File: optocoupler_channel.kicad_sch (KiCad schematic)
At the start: 22 parts, among them Q1 MMBT5551 200-300, Q2 MMBT5551 200-300, Q3 MMBT5401 200-300, Q4 MMBT5551 200-300, Q5 MMBT5551 200-300, U3 LTV-217-B-G, U5 LTV-217-B-G, U6 LTV-217-B-G

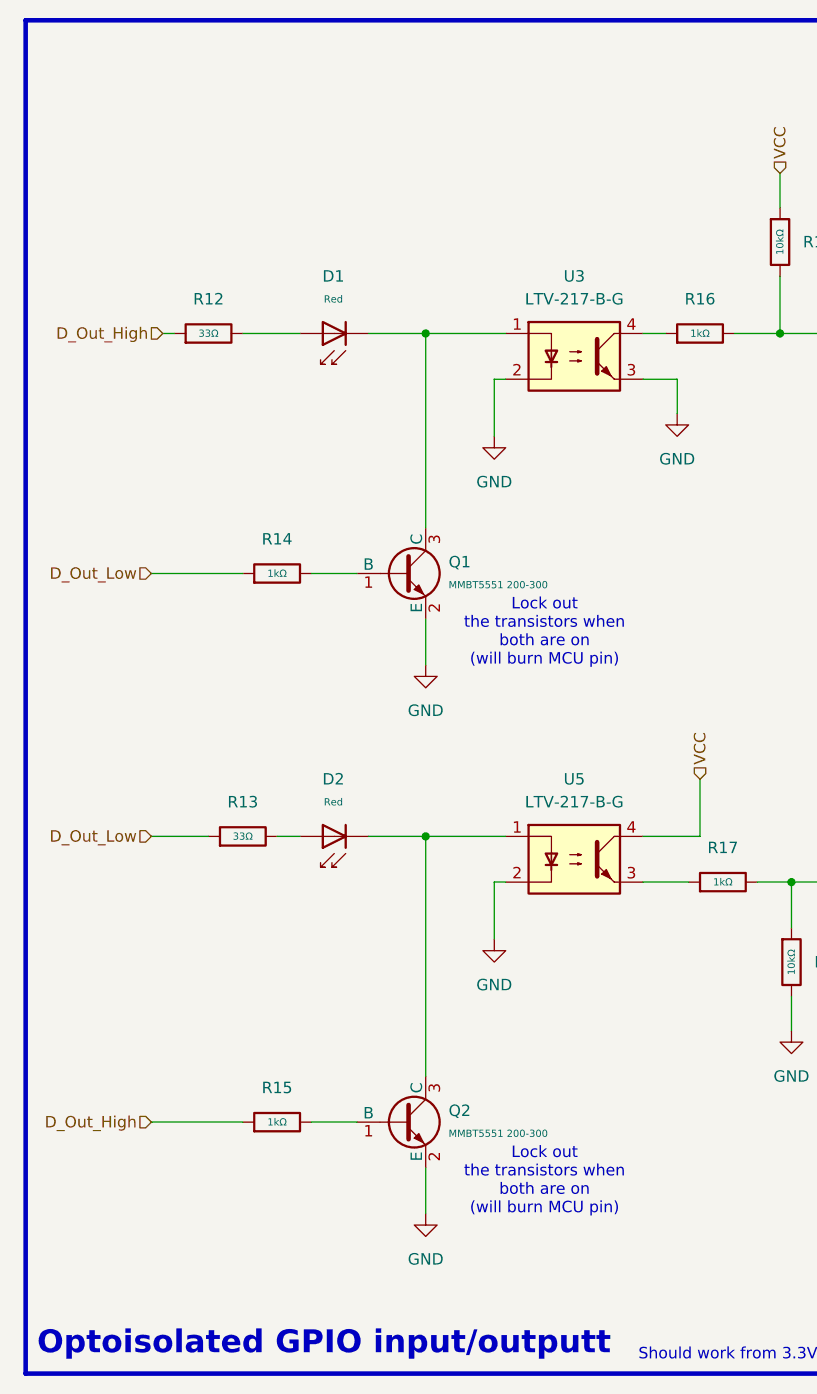
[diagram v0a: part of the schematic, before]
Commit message: routing impossible
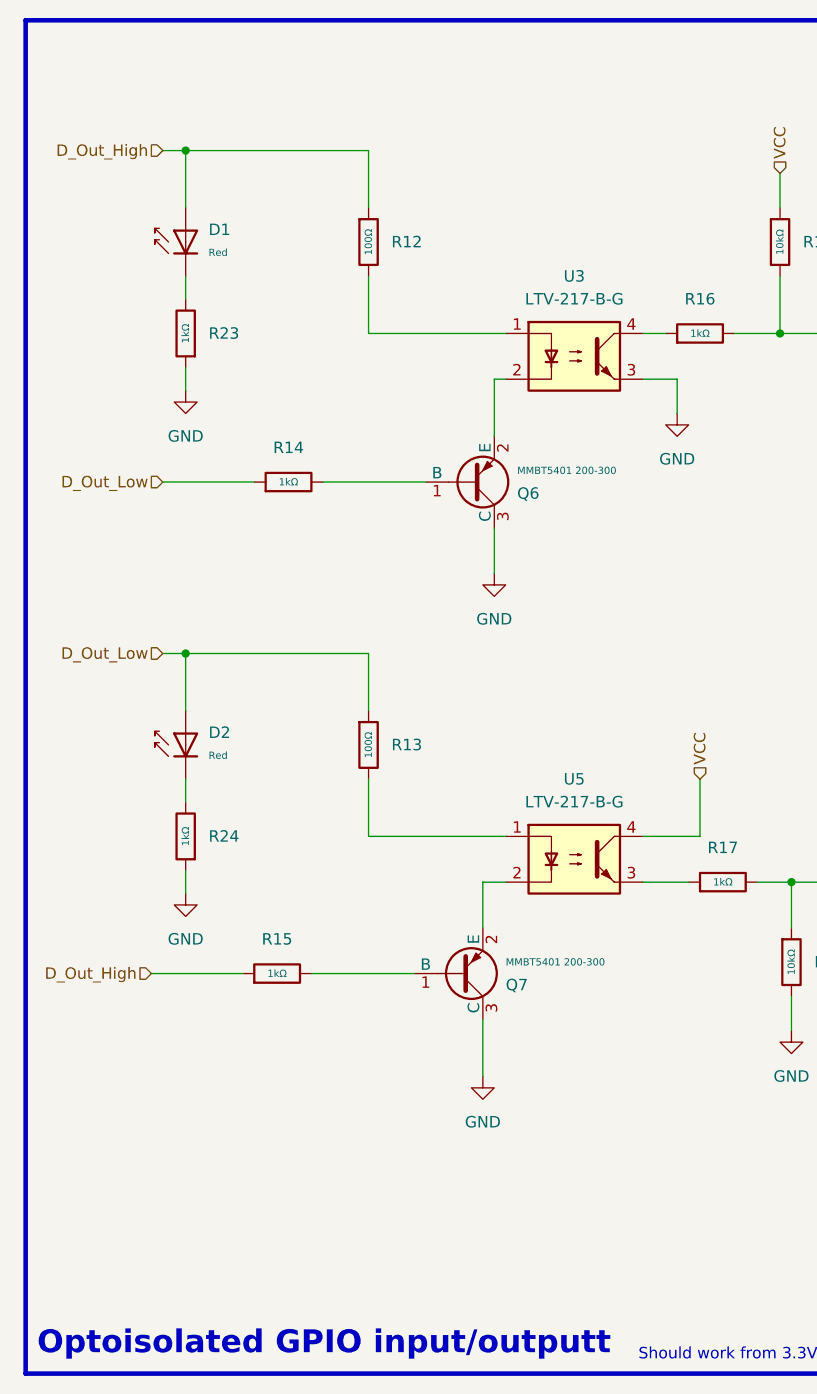
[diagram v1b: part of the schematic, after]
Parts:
- removed Q1, Q2: MMBT5551 200-300, PCM_JLCPCB:Q_SOT-23, symbol PCM_JLCPCB-Transistors:NPN,MMBT5551 200-300
- removed R12, R13: 33Ω, PCM_JLCPCB:R_0603, symbol PCM_JLCPCB-Resistors:0603,33Ω
- added Q6, Q7: MMBT5401 200-300, PCM_JLCPCB:Q_SOT-23, symbol PCM_JLCPCB-Transistors:PNP,MMBT5401 200-300
- added R12, R13: 100Ω, PCM_JLCPCB:R_0603, symbol PCM_JLCPCB-Resistors:0603,100Ω
- added R23, R24: 1kΩ, PCM_JLCPCB:R_0603, symbol PCM_JLCPCB-Resistors:0603,1kΩ
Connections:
- net D_Out_High: now also D1.2, R12.1
- net D_Out_Low: now also D2.2, R13.1
- net GND: now also Q6.3 (C), Q7.3 (C), R23.1, R24.1; no longer U3.2, U5.2
- net at R15.2: now also Q7.1 (B)
- net at U5.1: now also R13.2; no longer D2.1
- net at D1.1: now also R23.2; no longer U3.1
- net at R14.2: now also Q6.1 (B)
- new net: Q7.2 (E), U5.2
- new net: R12.2, U3.1
- new net: Q6.2 (E), U3.2
- new net: D2.1, R24.2
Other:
- note removed: "Lock out the transistors when both are on (will burn MCU pin)"
- moved on the sheet: R14
